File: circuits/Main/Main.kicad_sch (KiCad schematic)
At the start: 42 parts, among them J16 Conn_01x07_Socket, J7 Conn_01x07_Female, J8 Conn_01x10_Male, SW2 SW_SPST, SW3 SW_SPST, SW4 SW_SPST, SW5 SW_SPST, U12 STM32F446VETx, U13 TWE-L-WX, U14 BNO055, Y1 16MHz, Y2 32.768kHz

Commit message: こみっと
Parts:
- removed C21, C22, C23: 22pF, Capacitor_SMD:C_0603_1608Metric, symbol Device:C
- removed C25, C26, C27, C28, C29, C30, C33, C36: 0.1uF, Capacitor_SMD:C_0402_1005Metric, symbol Device:C
- removed C32: 1uF, Capacitor_SMD:C_0402_1005Metric, symbol Device:C
- removed D10, D8, D9: Red, LED_SMD:LED_0603_1608Metric_Pad1.05x0.95mm_HandSolder, symbol Device:LED
- removed J16: Conn_01x07_Socket, Connector_PinSocket_2.54mm:PinSocket_1x07_P2.54mm_Vertical, symbol Connector:Conn_01x07_Socket
- removed J7: Conn_01x07_Female, Connector_PinSocket_2.54mm:PinSocket_1x07_P2.54mm_Horizontal, symbol Connector:Conn_01x07_Female
- removed J8: Conn_01x10_Male, MyLibrary:BoxHeader_2x05_P1.27mm_Horizontal, symbol Connector:Conn_01x10_Male
- removed R71: 10k, Resistor_SMD:R_0402_1005Metric, symbol Device:R
- removed R73, R74, R78: PullUP?, Resistor_SMD:R_0603_1608Metric, symbol Device:R
- removed R76, R77: 1k, Resistor_SMD:R_0402_1005Metric, symbol Device:R
- removed R79, R80: PullUP, Resistor_SMD:R_0603_1608Metric_Pad0.98x0.95mm_HandSolder, symbol Device:R
- removed SW2, SW3: SW_SPST, Button_Switch_SMD:SW_Push_1P1T_NO_Vertical_Wuerth_434133025816, symbol Switch:SW_SPST
- removed U13: TWE-L-WX, RF_Module:MonoWireless_TWE-L-WX, symbol RF_ZigBee:TWE-L-WX
- removed U14: BNO055, MyLibrary:Sensor_Motion_Aktk_BNO055, symbol Sensor_Motion:BNO055
- removed Y1: 16MHz, Crystal:Crystal_SMD_3225-4Pin_3.2x2.5mm_HandSoldering, symbol Device:Crystal_GND24
- removed Y2: 32.768kHz, Crystal:Crystal_SMD_3215-2Pin_3.2x1.5mm, symbol Device:Crystal
- added C19: 1uF, Capacitor_SMD:C_0402_1005Metric, symbol Device:C
- added C20, C43, C44, C45, C46: 0.1uF, Capacitor_SMD:C_0402_1005Metric, symbol Device:C
- added C39, C40, C41, C42: 22pF, Capacitor_SMD:C_0603_1608Metric, symbol Device:C
- added J7: Conn_01x14_Pin, symbol Connector:Conn_01x14_Pin
- added Y3: 16MHz, Crystal:Crystal_SMD_3225-4Pin_3.2x2.5mm_HandSoldering, symbol Device:Crystal_GND24
- added Y4: 32.768kHz, Crystal:Crystal_SMD_3215-2Pin_3.2x1.5mm, symbol Device:Crystal
- C24: value 22pF -> 0.1uF; footprint Capacitor_SMD:C_0603_1608Metric -> Capacitor_SMD:C_0402_1005Metric
- C34: value 1uF -> 0.1uF
- R75: value 1k -> 10k
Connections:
- net PRG is gone; now on net NRST: SW5.1 (A)
- net Twe_LED0 is gone; now on net GNDD: R75.2
- net +3.3V: now also C24.1, C34.1, D7.2 (A), SW4.2 (B), U12.100 (VDD), U12.11 (VDD), U12.19 (VDD), U12.22 (VDDA), U12.28 (VDD), U12.50 (VDD), U12.6 (VBAT), U12.75 (VDD), C19.1, C20.1, C43.1, C44.1, C45.1; no longer C34.2
- net BOOT0: now also R75.1, SW4.1 (A)
- net GND: no longer C24.1, C34.1, C35.2, R72.2, SW4.2 (B), SW5.2 (B)
- net HSE_IN: now also C39.2, Y3.1
- net HSE_OUT: now also C40.2, Y3.3
- net LSE_IN: now also C41.2, Y4.2
- net LSE_OUT: now also C42.2, Y4.1; no longer C24.2
- net NRST: now also C46.1, J7.12 (Pin_12)
- net SWO: now also J7.8 (Pin_8)
- net TweRST_Sig: no longer D7.1 (K)
- net GNDD: now reaches U12.10 (VSS), U12.27 (VSS), U12.49 (VSS), U12.74 (VSS), U12.99 (VSS)
- net GNDD: now also C24.2, C34.2, C35.2, R72.2, SW5.2 (B), U12.20 (VSSA), C19.2, C20.2, C39.1, C40.1, C41.1, C42.1, C43.2, C44.2, C45.2, C46.2, J7.11 (Pin_11), J7.5 (Pin_5), J7.7 (Pin_7), Y3.2, Y3.4
- removed net RST: D7.2 (A), SW4.1 (A)
- new net SWCLK: J7.6 (Pin_6)
- new net SWDIO: J7.4 (Pin_4)
- new net VBUS: D7.1 (K), J7.3 (Pin_3)
- no-connect marks 12 -> 6
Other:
- added sheet BNO055 (BNO055.kicad_sch)
- added sheet Mouse (Mouse.kicad_sch)
- added sheet TweLite (TweLite.kicad_sch)
- added sheet UI (UI.kicad_sch)
- sheet Power ports: added V_Meas.; removed none
- sheet RS485 ports: added MainRX_RS485Bst_TX, MainRX_RS485Cam_TX, MainRX_RS485MD_TX, MainRX_RS485Spr_TX, MainRX_RS485UI_TX, MainTX_RS485Bst_RX, MainTX_RS485Cam_RX, MainTX_RS485MD_RX, MainTX_RS485Spr_RX, MainTX_RS485UI_RX; removed none
- note added: "F446VE"
- note added: "マウスセンサー"
- note added: "書き込み"
- note removed: "BNO055"
- note removed: "F446RE"
- note removed: "LED"
- note removed: "PRG"
- note removed: "TweLite"
- note removed: "TweLiteR3"
- note removed: "リセット"
- moved on the sheet: C31, R72, U12

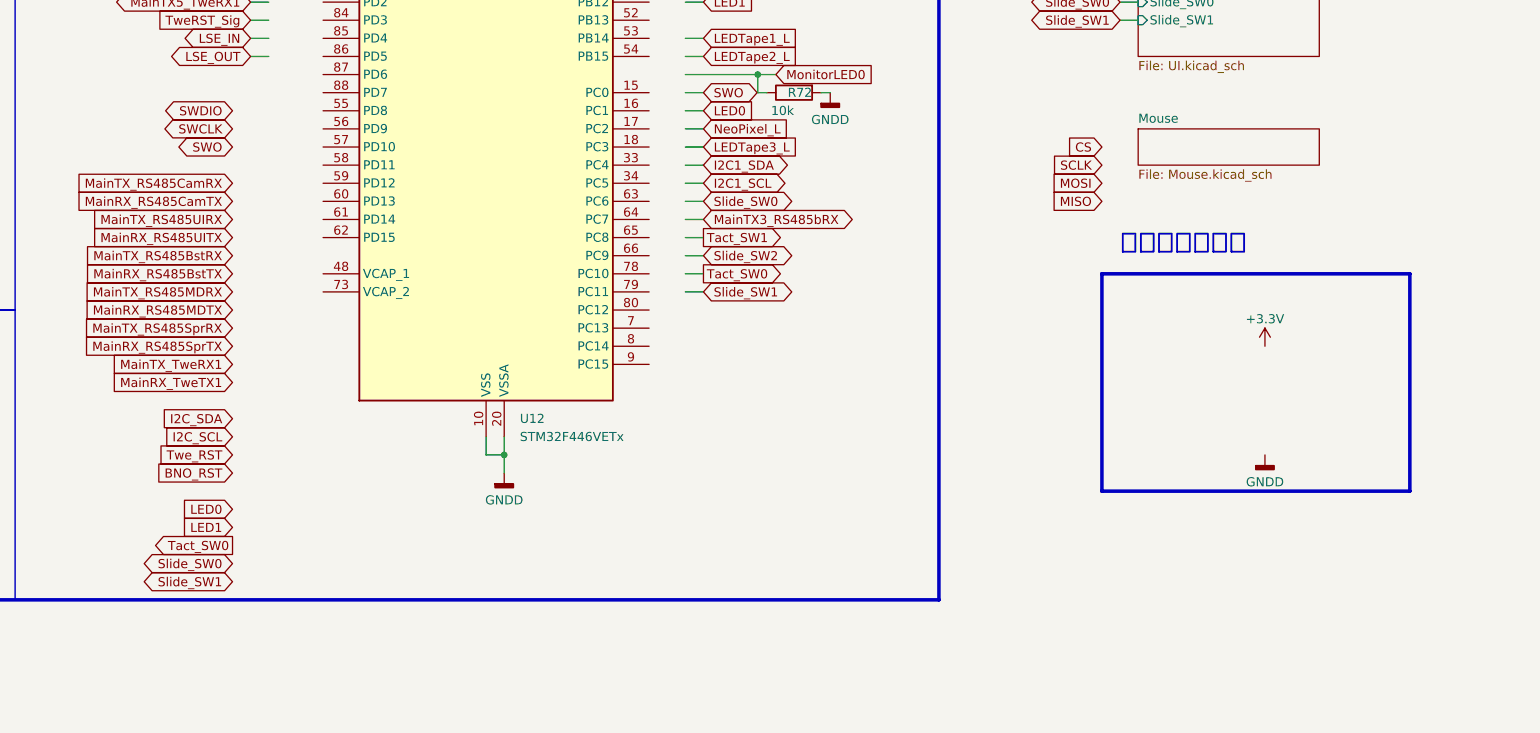
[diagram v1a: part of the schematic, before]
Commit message: とちゅう
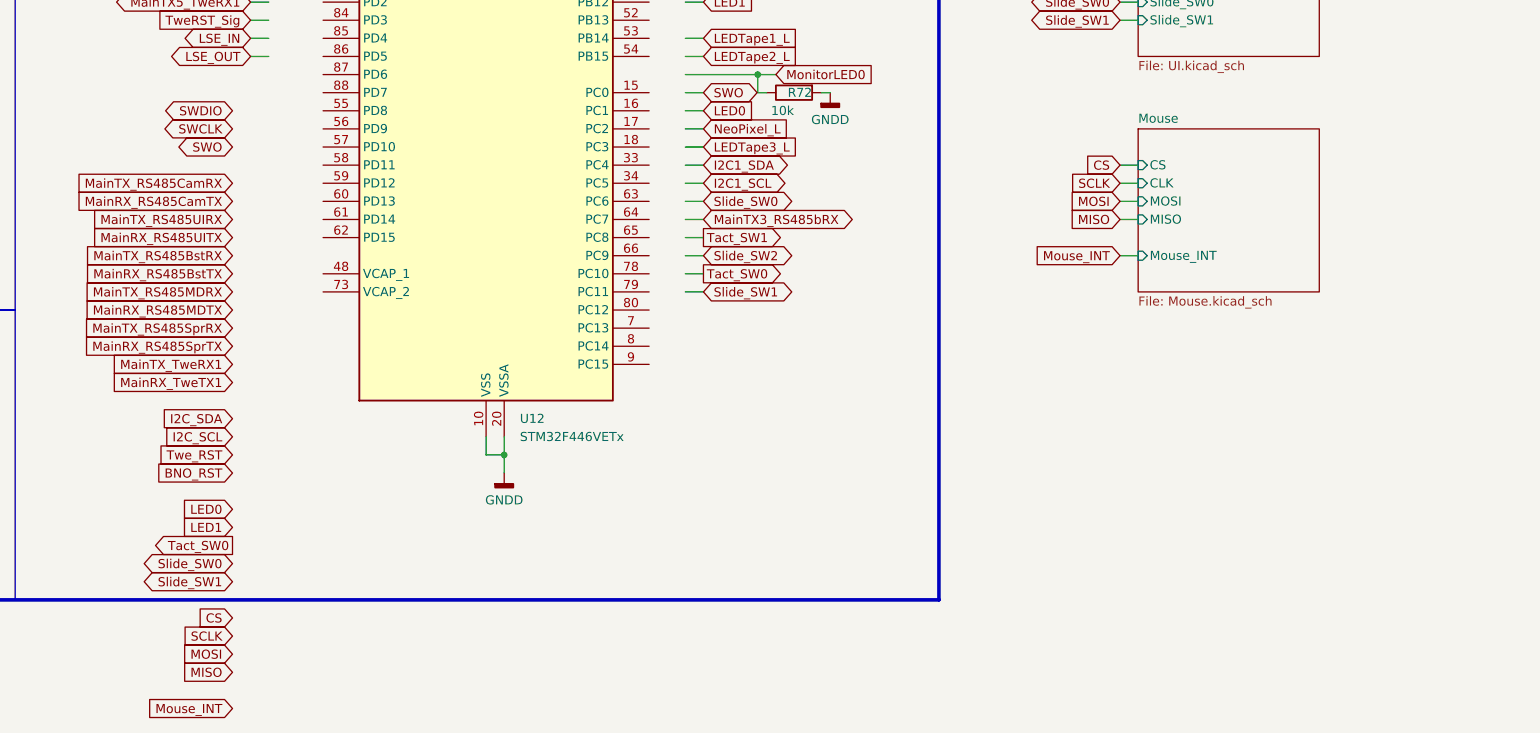
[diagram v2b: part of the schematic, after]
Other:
- sheet Mouse ports: added CLK, CS, MISO, MOSI, Mouse_INT; removed none
- note removed: "マウスセンサー"
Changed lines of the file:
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@@
     (stroke (width 0) (type default))
-  )
-  (polyline (pts (xy 304.8 241.3) (xy 261.62 241.3))
-    (stroke (width 0.5) (type default))
   )
   (wire (pts (xy 264.16 111.76) (xy 266.7 111.76))
     (stroke (width 0) (type default))
   )
+  (wire (pts (xy 264.16 203.2) (xy 266.7 203.2))
+    (stroke (width 0) (type default))
+  )
   (wire (pts (xy 81.28 181.61) (xy 81.28 182.88))
     (stroke (width 0) (type default))
@@
   (wire (pts (xy 182.88 93.98) (xy 182.88 91.44))
     (stroke (width 0) (type default))
-  )
-  (polyline (pts (xy 304.8 210.82) (xy 304.8 241.3))
-    (stroke (width 0.5) (type default))
   )
   (wire (pts (xy 264.16 132.08) (xy 266.7 132.08))
@@
     (stroke (width 0) (type solid))
   )
-  (polyline (pts (xy 261.62 210.82) (xy 304.8 210.82))
-    (stroke (width 0.5) (type default))
-  )
   (wire (pts (xy 71.12 233.68) (xy 78.74 233.68))
     (stroke (width 0) (type default))
@@
     (stroke (width 0) (type default))
   )
-  (polyline (pts (xy 261.62 241.3) (xy 261.62 210.82))
-    (stroke (width 0.5) (type default))
-  )
   (wire (pts (xy 81.28 193.04) (xy 81.28 187.96))
     (stroke (width 0) (type default))
@@
   )
   (wire (pts (xy 264.16 162.56) (xy 266.7 162.56))
+    (stroke (width 0) (type default))
+  )
+  (wire (pts (xy 264.16 195.58) (xy 266.7 195.58))
     (stroke (width 0) (type default))
   )
@@
     (stroke (width 0) (type default))
   )
+  (wire (pts (xy 264.16 200.66) (xy 266.7 200.66))
+    (stroke (width 0) (type default))
+  )
   (wire (pts (xy 264.16 175.26) (xy 266.7 175.26))
     (stroke (width 0) (type default))
@@
     (stroke (width 0) (type default))
   )
+  (wire (pts (xy 264.16 208.28) (xy 266.7 208.28))
+    (stroke (width 0) (type default))
+  )
   (wire (pts (xy 142.24 175.26) (xy 144.78 175.26))
     (stroke (width 0) (type default))
@@
     (stroke (width 0) (type default))
   )
+  (wire (pts (xy 264.16 198.12) (xy 266.7 198.12))
+    (stroke (width 0) (type default))
+  )
   (rectangle (start 35.56 215.9) (end 109.22 215.9)
     (stroke (width 0) (type default))
@@
     (effects (font (size 1.27 1.27)) (justify left bottom))
   )
-  (text "マウスセンサー" (at 264.16 208.28 0)
-    (effects (font (size 2.54 2.54) (thickness 0.254) bold) (justify left bottom))
-  )
   (text "LSE" (at 38.1 109.22 0)
     (effects (font (size 1.27 1.27)) (justify left bottom))
@@
     )
   )
+  (global_label "Mouse_INT" (shape input) (at 264.16 208.28 180) (fields_autoplaced)
+    (effects (font (size 1.27 1.27)) (justify right))
+    (property "Intersheetrefs" "${INTERSHEET_REFS}" (at 251.4382 208.28 0)
+      (effects (font (size 1.27 1.27)) (justify right) hide)
+    )
+  )
   (global_label "MainRX5_TweTX1" (shape bidirectional) (at 142.24 137.16 180) (fields_autoplaced)
     (effects (font (size 1.27 1.27)) (justify right))
@@
     )
   )
+  (global_label "Mouse_INT" (shape input) (at 139.7 271.78 180) (fields_autoplaced)
+    (effects (font (size 1.27 1.27)) (justify right))
+    (property "Intersheetrefs" "${INTERSHEET_REFS}" (at 126.9782 271.78 0)
+      (effects (font (size 1.27 1.27)) (justify right) hide)
+    )
+  )
   (global_label "MainTX_RS485SprRX" (shape input) (at 139.7 218.44 180) (fields_autoplaced)
     (effects (font (size 1.27 1.27)) (justify right))
@@
     )
   )
+  (global_label "MISO" (shape input) (at 139.7 266.7 180) (fields_autoplaced)
+    (effects (font (size 1.27 1.27)) (justify right))
+    (property "Intersheetrefs" "${INTERSHEET_REFS}" (at 132.1186 266.7 0)
+      (effects (font (size 1.27 1.27)) (justify right) hide)
+    )
+  )
   (global_label "MainRX_RS485UITX" (shape input) (at 139.7 205.74 180) (fields_autoplaced)
     (effects (font (size 1.27 1.27)) (justify right))
@@
     )
   )
-  (global_label "MOSI" (shape input) (at 261.62 198.12 180) (fields_autoplaced)
-    (effects (font (size 1.27 1.27)) (justify right))
-    (property "Intersheetrefs" "${INTERSHEET_REFS}" (at 254.0386 198.12 0)
+  (global_label "MOSI" (shape input) (at 264.16 200.66 180) (fields_autoplaced)
+    (effects (font (size 1.27 1.27)) (justify right))
+    (property "Intersheetrefs" "${INTERSHEET_REFS}" (at 256.5786 200.66 0)
       (effects (font (size 1.27 1.27)) (justify right) hide)
     )
@@
     )
   )
-  (global_label "CS" (shape input) (at 261.62 193.04 180) (fields_autoplaced)
-    (effects (font (size 1.27 1.27)) (justify right))
-    (property "Intersheetrefs" "${INTERSHEET_REFS}" (at 256.1553 193.04 0)
+  (global_label "CS" (shape input) (at 264.16 195.58 180) (fields_autoplaced)
+    (effects (font (size 1.27 1.27)) (justify right))
+    (property "Intersheetrefs" "${INTERSHEET_REFS}" (at 258.6953 195.58 0)
       (effects (font (size 1.27 1.27)) (justify right) hide)
     )
@@
     )
   )
-  (global_label "SCLK" (shape input) (at 261.62 195.58 180) (fields_autoplaced)
-    (effects (font (size 1.27 1.27)) (justify right))
-    (property "Intersheetrefs" "${INTERSHEET_REFS}" (at 253.8572 195.58 0)
+  (global_label "SCLK" (shape input) (at 264.16 198.12 180) (fields_autoplaced)
+    (effects (font (size 1.27 1.27)) (justify right))
+    (property "Intersheetrefs" "${INTERSHEET_REFS}" (at 256.3972 198.12 0)
       (effects (font (size 1.27 1.27)) (justify right) hide)
     )
@@
     )
   )
-  (global_label "MISO" (shape input) (at 261.62 200.66 180) (fields_autoplaced)
-    (effects (font (size 1.27 1.27)) (justify right))
-    (property "Intersheetrefs" "${INTERSHEET_REFS}" (at 254.0386 200.66 0)
+  (global_label "MISO" (shape input) (at 264.16 203.2 180) (fields_autoplaced)
+    (effects (font (size 1.27 1.27)) (justify right))
+    (property "Intersheetrefs" "${INTERSHEET_REFS}" (at 256.5786 203.2 0)
       (effects (font (size 1.27 1.27)) (justify right) hide)
     )
@@
     )
   )
+  (global_label "MOSI" (shape input) (at 139.7 264.16 180) (fields_autoplaced)
+    (effects (font (size 1.27 1.27)) (justify right))
+    (property "Intersheetrefs" "${INTERSHEET_REFS}" (at 132.1186 264.16 0)
+      (effects (font (size 1.27 1.27)) (justify right) hide)
+    )
+  )
   (global_label "Slide_SW0" (shape bidirectional) (at 139.7 251.46 180) (fields_autoplaced)
     (effects (font (size 1.27 1.27)) (justify right))
@@
     )
   )
+  (global_label "CS" (shape input) (at 139.7 259.08 180) (fields_autoplaced)
+    (effects (font (size 1.27 1.27)) (justify right))
+    (property "Intersheetrefs" "${INTERSHEET_REFS}" (at 134.2353 259.08 0)
+      (effects (font (size 1.27 1.27)) (justify right) hide)
+    )
+  )
   (global_label "MainTX_TweRX1" (shape input) (at 139.7 223.52 180) (fields_autoplaced)
     (effects (font (size 1.27 1.27)) (justify right))
@@
     (effects (font (size 1.27 1.27)) (justify right))
     (property "Intersheetrefs" "${INTERSHEET_REFS}" (at 117.907 213.36 0)
+      (effects (font (size 1.27 1.27)) (justify right) hide)
+    )
+  )
+  (global_label "SCLK" (shape input) (at 139.7 261.62 180) (fields_autoplaced)
+    (effects (font (size 1.27 1.27)) (justify right))
+    (property "Intersheetrefs" "${INTERSHEET_REFS}" (at 131.9372 261.62 0)
       (effects (font (size 1.27 1.27)) (justify right) hide)
     )
@@
         (path "/aa9d7141-7530-418f-853d-a56ee68433fb"
           (reference "C45") (unit 1)
-        )
-      )
-    )
-  )
-  (symbol (lib_id "power:GNDD") (at 284.48 236.22 0) (unit 1)
-    (in_bom yes) (on_board yes) (dnp no) (fields_autoplaced)
-    (property "Reference" "#PWR0137" (at 284.48 242.57 0)
-      (effects (font (size 1.27 1.27)) hide)
-    )
-    (property "Value" "GNDD" (at 284.48 240.03 0)
-      (effects (font (size 1.27 1.27)))
-    )
-    (property "Footprint" "" (at 284.48 236.22 0)
-      (effects (font (size 1.27 1.27)) hide)
-    )
-    (property "Datasheet" "" (at 284.48 236.22 0)
-      (effects (font (size 1.27 1.27)) hide)
-    )
-    (pin "1")
-    (instances
-      (project "Main"
-        (path "/aa9d7141-7530-418f-853d-a56ee68433fb"
-          (reference "#PWR0137") (unit 1)
         )
       )
@@
     )
   )
-  (symbol (lib_id "power:+3.3V") (at 284.48 220.98 0) (unit 1)
-    (in_bom yes) (on_board yes) (dnp no) (fields_autoplaced)
-    (property "Reference" "#PWR0111" (at 284.48 224.79 0)
-      (effects (font (size 1.27 1.27)) hide)
-    )
-    (property "Value" "+3.3V" (at 284.48 217.17 0)
-      (effects (font (size 1.27 1.27)))
-    )
-    (property "Footprint" "" (at 284.48 220.98 0)
-      (effects (font (size 1.27 1.27)) hide)
-    )
-    (property "Datasheet" "" (at 284.48 220.98 0)
-      (effects (font (size 1.27 1.27)) hide)
-    )
-    (pin "1")
-    (instances
-      (project "Main"
-        (path "/aa9d7141-7530-418f-853d-a56ee68433fb"
-          (reference "#PWR0111") (unit 1)
-        )
-      )
-    )
-  )
   (symbol (lib_id "power:GNDD") (at 157.48 91.44 0) (unit 1)
     (in_bom yes) (on_board yes) (dnp no)
@@
     )
   )
-  (sheet (at 266.7 190.5) (size 25.4 5.08) (fields_autoplaced)
+  (sheet (at 266.7 190.5) (size 25.4 22.86) (fields_autoplaced)
     (stroke (width 0.1524) (type solid))
     (fill (color 0 0 0 0.0000))
@@
       (effects (font (size 1.27 1.27)) (justify left bottom))
     )
-    (property "Sheetfile" "Mouse.kicad_sch" (at 266.7 196.1646 0)
+    (property "Sheetfile" "Mouse.kicad_sch" (at 266.7 213.9446 0)
       (effects (font (size 1.27 1.27)) (justify left top))
     )
-    (instances
+    (pin "CLK" input (at 266.7 198.12 180)
+      (effects (font (size 1.27 1.27)) (justify left))
+    )
+    (pin "CS" input (at 266.7 195.58 180)
+      (effects (font (size 1.27 1.27)) (justify left))
+    )
+    (pin "MISO" input (at 266.7 203.2 180)
+      (effects (font (size 1.27 1.27)) (justify left))
+    )
+    (pin "MOSI" input (at 266.7 200.66 180)
+      (effects (font (size 1.27 1.27)) (justify left))
+    )
+    (pin "Mouse_INT" input (at 266.7 208.28 180)
+      (effects (font (size 1.27 1.27)) (justify left))
+    )
+    (instances

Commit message: すてい
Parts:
- removed C41, C42: 22pF, Capacitor_SMD:C_0603_1608Metric, symbol Device:C
- removed J7: Conn_01x14_Pin, symbol Connector:Conn_01x14_Pin
- removed R72: 10k, Resistor_SMD:R_0402_1005Metric, symbol Device:R
- removed SW4: SW_SPST, Button_Switch_SMD:SW_Push_1P1T_NO_Vertical_Wuerth_434133025816, symbol Switch:SW_SPST
- removed Y4: 32.768kHz, Crystal:Crystal_SMD_3215-2Pin_3.2x1.5mm, symbol Device:Crystal
- added C27: 1uF, Capacitor_SMD:C_0402_1005Metric, symbol Device:C
- added C28, C29: 2.2uF, Capacitor_SMD:C_0402_1005Metric, symbol Device:C
- added J6: Conn_01x14_Pin, MyLibrary:BoxHeader_2x07_P1.27mm_Horizontal, symbol Connector:Conn_01x14_Pin
- added R64: 10k, Resistor_SMD:R_0402_1005Metric, symbol Device:R
- added R68: 1k, Resistor_SMD:R_0402_1005Metric, symbol Device:R
- C19: value 1uF -> 0.1uF
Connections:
- net GND is gone; now on net +3.3V: C31.1
- net +3.3V: now also U12.21 (VREF+), C27.1; no longer C19.1
- net BOOT0: now also U12.94 (BOOT0)
- net DAC: now also C19.1, U12.29 (PA4), R68.2
- net GNDD: now also C31.2, C27.2, C28.2, C29.2, J6.11 (Pin_11), J6.5 (Pin_5), J6.7 (Pin_7), R64.2, R68.1
- net HSE_IN: now also U12.12 (PH0)
- net HSE_OUT: now also U12.13 (PH1)
- net I2C1_SCL: now also U12.92 (PB6)
- net I2C1_SDA: now also U12.93 (PB7)
- net NRST: now also U12.14 (NRST), J6.12 (Pin_12)
- net SWCLK: now also U12.76 (PA14), J6.6 (Pin_6)
- net SWDIO: now also U12.72 (PA13), J6.4 (Pin_4)
- net SWO: now also U12.89 (PB3), J6.8 (Pin_8)
- net VBUS: now also J6.3 (Pin_3)
- net MainRX4_RS485TX: now reaches U12.24 (PA1)
- net MainTX2_RS485RX: now reaches U12.25 (PA2)
- net MainRX2_RS485TX: now reaches U12.26 (PA3)
- net at U12.37 (PB2): now also R64.1
- net MainRX5_RS485TX: now reaches U12.38 (PE7)
- net MainTX5_RS485RX: now reaches U12.39 (PE8)
- net at U12.48 (VCAP_1): now also C28.1
- net at U12.73 (VCAP_2): now also C29.1
- no-connect marks 6 -> 11
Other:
- note added: "マイコン側のラベルと階層シート側のラベルをそれぞれ対応するように書き換える"
- note removed: "LSE"
- moved on the sheet: C31, C39, C40, Y3

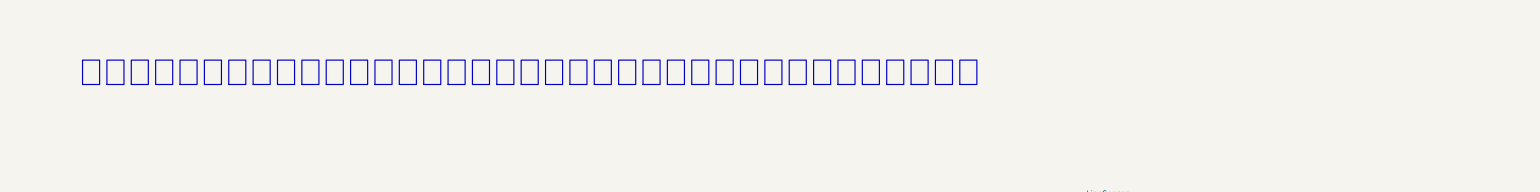
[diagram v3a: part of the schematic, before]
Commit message: 修正
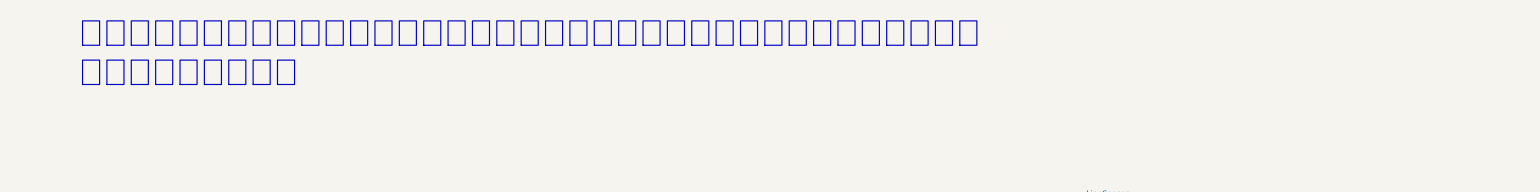
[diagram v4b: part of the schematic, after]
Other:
- note added: "マイコン側のラベルと階層シート側のラベルをそれぞれ対応するように書き換える 電解コンの耐圧注意"
- note removed: "マイコン側のラベルと階層シート側のラベルをそれぞれ対応するように書き換える"
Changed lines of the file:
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@@
     (effects (font (size 1.27 1.27)) (justify left bottom))
   )
-  (text "マイコン側のラベルと階層シート側のラベルをそれぞれ対応するように書き換える" (at 124.46 30.48 0)
+  (text "マイコン側のラベルと階層シート側のラベルをそれぞれ対応するように書き換える\n電解コンの耐圧注意" (at 124.46 30.48 0)
     (effects (font (size 5.56 5.56)) (justify left bottom))
   )
